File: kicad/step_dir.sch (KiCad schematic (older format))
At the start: 16 parts, among them J1001 tblock2x6, U1001 am26ls32a

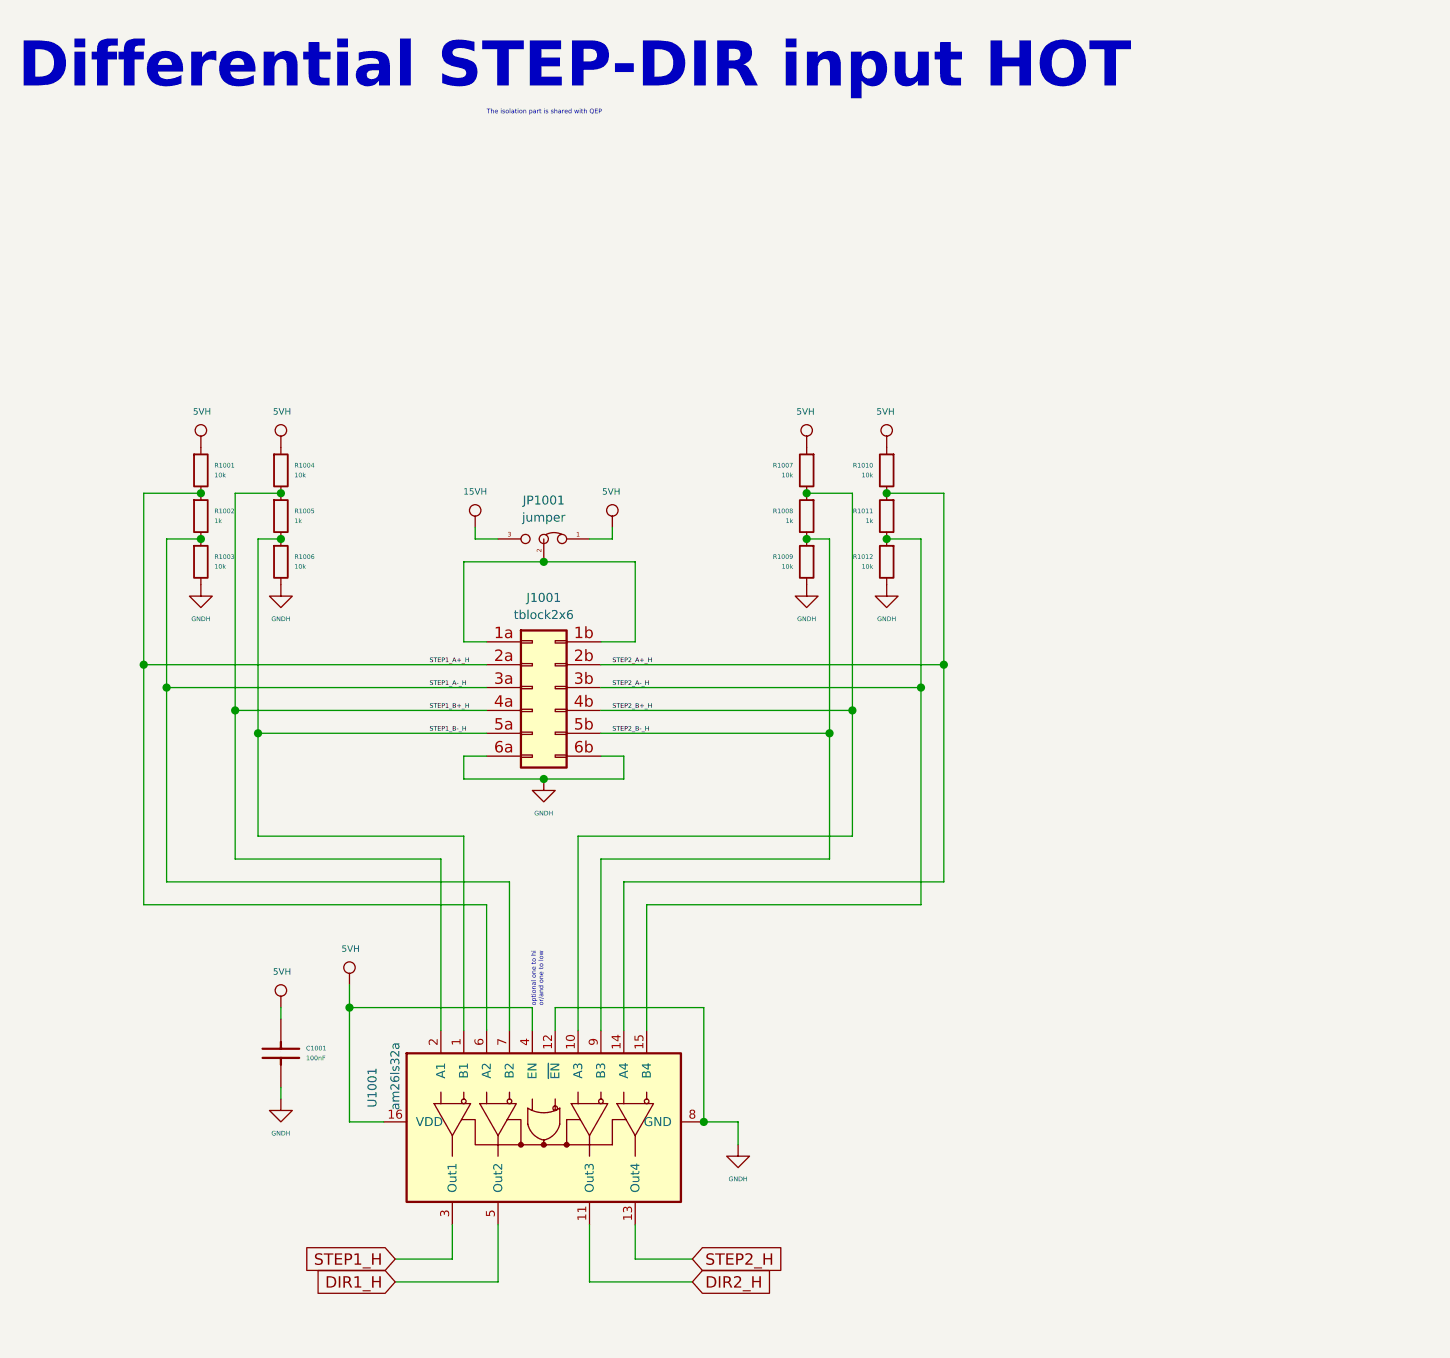
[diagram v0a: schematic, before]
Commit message: touting....
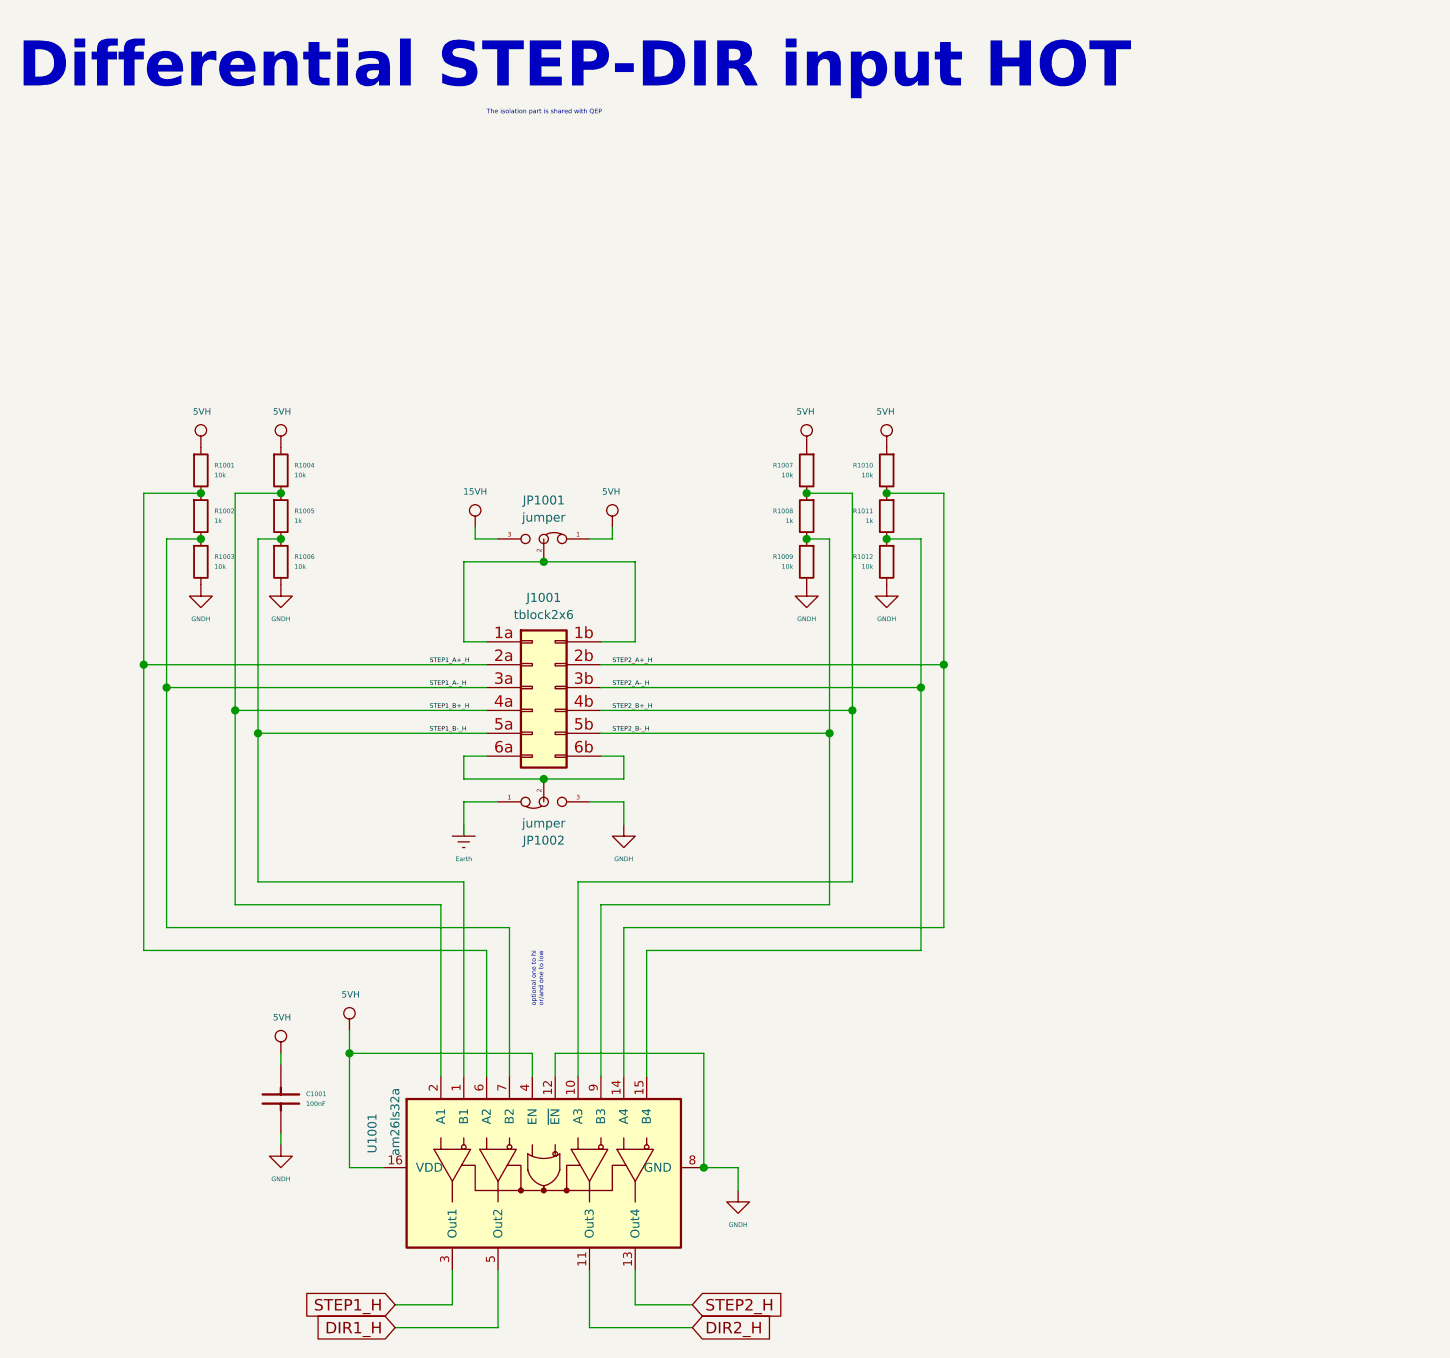
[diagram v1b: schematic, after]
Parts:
- added JP1002: jumper, Jumper:SolderJumper-3_P1.3mm_Open_RoundedPad1.0x1.5mm, symbol servo:Jumper_3_Bridged12
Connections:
- net GNDH: now also JP1002.3 (B); no longer J1001.6a (Pin_6a), J1001.6b (Pin_6b)
- new net: J1001.6a (Pin_6a), J1001.6b (Pin_6b), JP1002.2 (C)
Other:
- moved on the sheet: C1001, U1001
